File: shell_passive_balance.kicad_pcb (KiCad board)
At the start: 4 copper layers, 58.9 x 66.3 mm, 51 parts, among them J1 Conn_01x20_Pin, J2 Conn_01x20_Pin, Q1 PMOS, Q10 PMOS, Q11 PMOS, Q12 PMOS, Q13 PMOS, Q14 PMOS, Q15 PMOS, Q16 PMOS, Q2 PMOS, Q3 PMOS, Q4 PMOS, Q5 PMOS, Q6 PMOS, Q7 PMOS, Q8 PMOS, Q9 PMOS

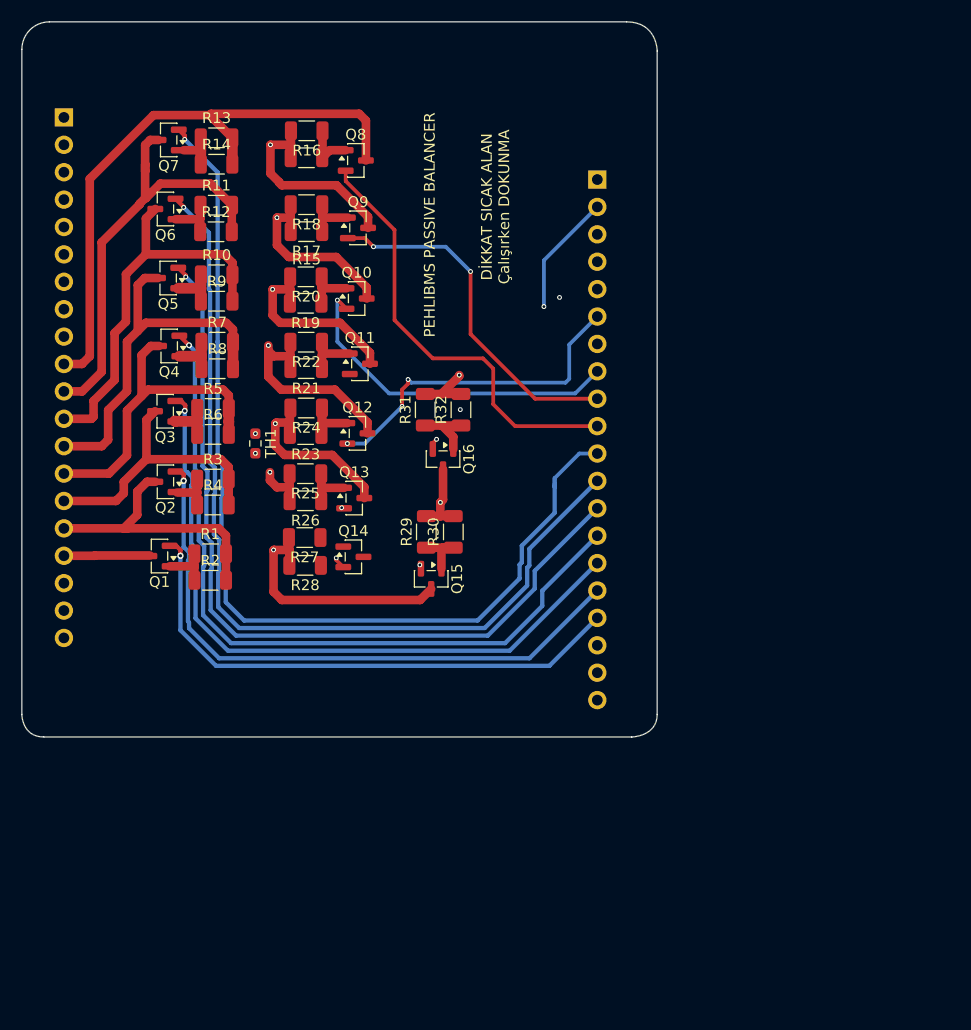
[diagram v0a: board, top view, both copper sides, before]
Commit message: finalised product
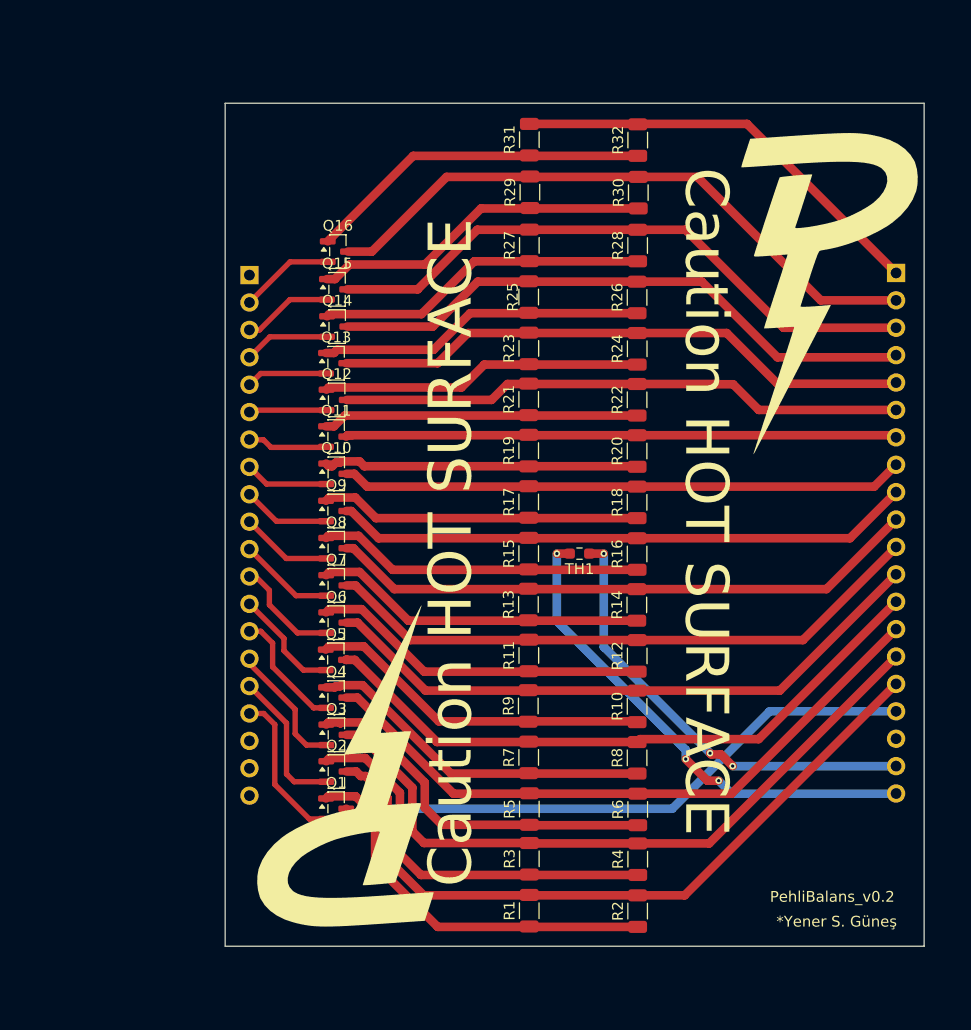
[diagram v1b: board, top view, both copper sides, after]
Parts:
- added G***: LOGO, LOGO, F.Cu at (194.1, 83.3)
- added G***: LOGO, LOGO, F.Cu at (150.7, 126.5)
- moved J2 78.5 mm to (201.0, 81.1)
- moved R14 56.5 mm to (177.0, 111.9), turned to 90 degrees
- moved R10 55.9 mm to (177.0, 121.3), turned to 90 degrees
- moved R12 55.4 mm to (177.0, 116.6), turned to 90 degrees
- moved R8 53.1 mm to (177.0, 126.0), turned to 90 degrees
- moved R6 52.5 mm to (177.1, 130.8), turned to 90 degrees
- moved R13 52.0 mm to (166.9, 111.8), turned to 90 degrees
- moved R4 51.3 mm to (177.1, 135.4), turned to 90 degrees
- moved R11 50.8 mm to (166.9, 116.5), turned to 90 degrees
- moved R2 50.1 mm to (177.0, 140.2), turned to 90 degrees
- moved R16 49.8 mm to (177.0, 107.1), turned to 90 degrees
- moved R7 48.1 mm to (166.9, 126.0), turned to 90 degrees
- moved R9 47.4 mm to (166.9, 121.2), turned to 90 degrees
- moved R5 47.3 mm to (167.0, 130.8), turned to 90 degrees
- moved R3 45.8 mm to (167.0, 135.4), turned to 90 degrees
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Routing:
- net /CI_10: track 91.7 -> 8.90 mm, vias 1 -> 0
- net /CI_11: track 83.1 -> 10.1 mm, vias 1 -> 0
- net /CI_12: track 75.8 -> 10.3 mm, vias 1 -> 0
- net /CI_13: track 69.6 -> 11.3 mm, vias 1 -> 0
- net /CI_14: track 63.5 -> 12.0 mm, vias 1 -> 0
- net /B_2: track 105.5 -> 56.9 mm, vias 1 -> 0
- net /B_16: track 7.99 -> 56.1 mm, vias 0 -> 1
- net /CI_15: track 57.0 -> 13.6 mm, vias 1 -> 0
- net /B_15: track 25.4 -> 67.1 mm
- net /B_14: track 26.1 -> 64.7 mm
- net /CI_16: track 50.5 -> 14.4 mm, vias 1 -> 0
- net Net-(Q2-D): track 4.24 -> 36.8 mm
- net /CI_9: track 40.7 -> 8.52 mm
- net Net-(Q1-D): track 5.10 -> 36.6 mm
- net Net-(Q14-D): track 0.00 -> 30.9 mm
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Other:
- board size 58.9 x 66.3 mm -> 64.8 x 78.2 mm
- board text added: "*Yener S. Güneş"
- board text added: "Caution HOT SURFACE"
- board text added: "Designed By anshinx* FOR SEM 2026"
- board text added: "PehliBalans_v0.2"
- board text added: "SEM2026"
- board text removed: "DİKKAT SICAK ALAN Çalışırken DOKUNMA"
- board text removed: "PEHLIBMS PASSIVE BALANCER"
